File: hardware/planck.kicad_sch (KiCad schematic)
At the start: 100 parts, among them SW1 SW_Push, SW10 SW_Push, SW11 SW_Push, SW12 SW_Push, SW13 SW_Push, SW14 SW_Push, SW15 SW_Push, SW16 SW_Push, SW17 SW_Push, SW18 SW_Push, SW19 SW_Push, SW2 SW_Push, SW20 SW_Push, SW21 SW_Push, SW22 SW_Push, SW23 SW_Push, SW24 SW_Push, SW25 SW_Push, SW26 SW_Push, SW27 SW_Push, SW28 SW_Push, SW29 SW_Push, SW3 SW_Push, SW30 SW_Push, SW31 SW_Push, SW32 SW_Push, SW33 SW_Push, SW34 SW_Push, SW35 SW_Push, SW36 SW_Push, SW37 SW_Push, SW38 SW_Push, SW39 SW_Push, SW4 SW_Push, SW40 SW_Push, SW41 SW_Push, SW42 SW_Push, SW43 SW_Push, SW44 SW_Push, SW45 SW_Push, SW46 SW_Push, SW47 SW_Push, SW48 SW_Push, SW5 SW_Push, SW6 SW_Push, SW7 SW_Push, SW8 SW_Push, SW9 SW_Push, U1 STM32F103CBTx, U2 AMS1117-3.3, Y1 Crystal

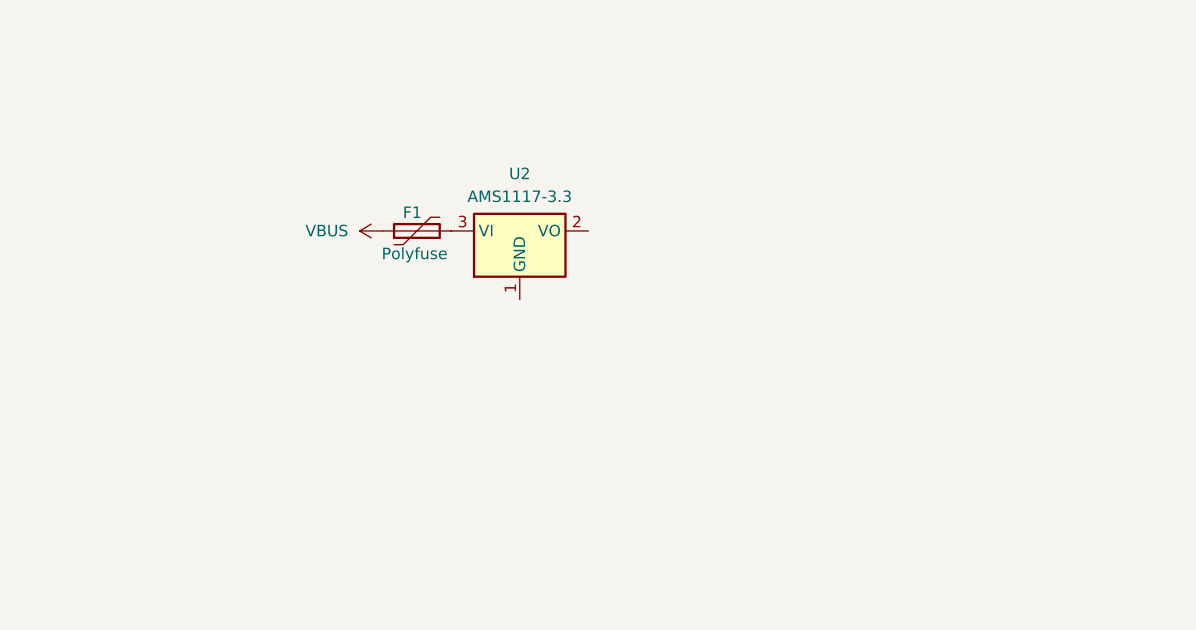
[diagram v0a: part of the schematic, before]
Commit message: feat: 电源第一版
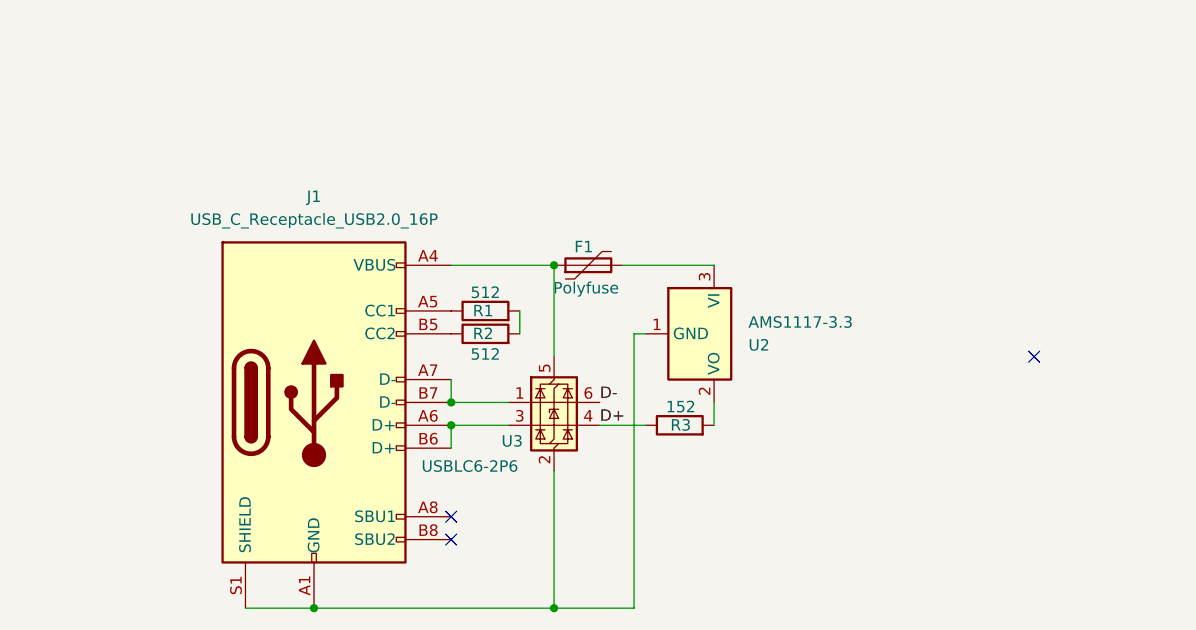
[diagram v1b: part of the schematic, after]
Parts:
- added J1: USB_C_Receptacle_USB2.0_16P, symbol Connector:USB_C_Receptacle_USB2.0_16P
- added R1, R2: 512, symbol Device:R
- added R3: 152, symbol Device:R
- added U3: USBLC6-2P6, Package_TO_SOT_SMD:SOT-666, symbol Power_Protection:USBLC6-2P6
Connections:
- net at U2.1 (GND): now also J1.A1 (GND), J1.A12 (GND), J1.B1 (GND), J1.B12 (GND), J1.S1 (SHIELD), U3.2 (GND)
- net at U2.2 (VO): now also R3.2
- net VBUS: no longer names the net of F1.1
- net VBUS: now also J1.A4 (VBUS), J1.A9 (VBUS), J1.B4 (VBUS), J1.B9 (VBUS), U3.5 (VBUS)
- new net: J1.A7 (D-), J1.B7 (D-), U3.1 (I/O1)
- new net: J1.A6 (D+), J1.B6 (D+), U3.3 (I/O2)
- new net: J1.A5 (CC1), R1.1
- new net: R1.2, R2.2
- new net: J1.B5 (CC2), R2.1
- new net D+: R3.1, U3.4 (I/O2)
- new net D-: U3.6 (I/O1)
- no-connect marks 0 -> 3
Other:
- moved on the sheet: F1, U2
